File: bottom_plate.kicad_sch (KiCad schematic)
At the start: 27 parts, among them J42 Osc Out, J43 Conn_02x08_Odd_Even, J44 Conn_02x08_Odd_Even, J45 Conn_02x08_Odd_Even, J46 Conn_02x08_Odd_Even, J47 Conn_02x08_Odd_Even, J48 Select, J49 Select, J60 VCC, J61 VCC, J62 GND, J63 GND, J64 Conn_02x08_Odd_Even, J66 4017 Pins, J67 4017 Pins, J68 Conn_01x16, J73 Conn_02x20_Odd_Even, J74 Conn_02x20_Odd_Even, J75 Conn_02x20_Odd_Even, J76 Conn_02x20_Odd_Even, J77 Conn_02x20_Odd_Even, J78 Conn_02x20_Odd_Even, J79 Conn_02x20_Odd_Even, J80 Conn_02x20_Odd_Even, J81 Conn_02x20_Odd_Even, J85 Output, J86 Output

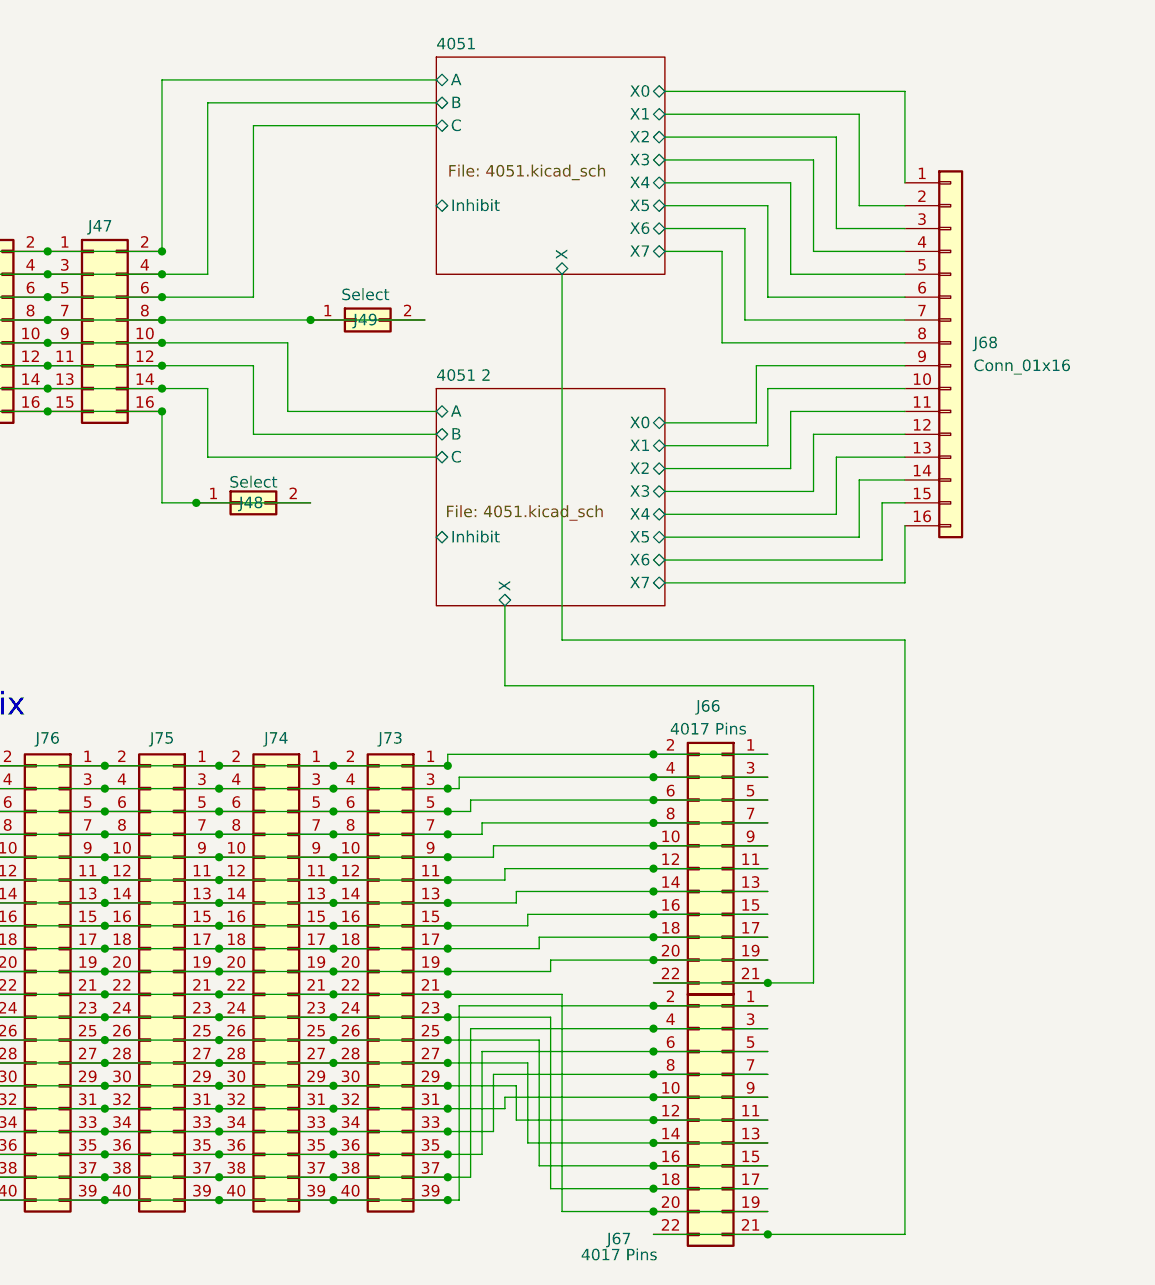
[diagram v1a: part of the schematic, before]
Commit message: 18x20 design
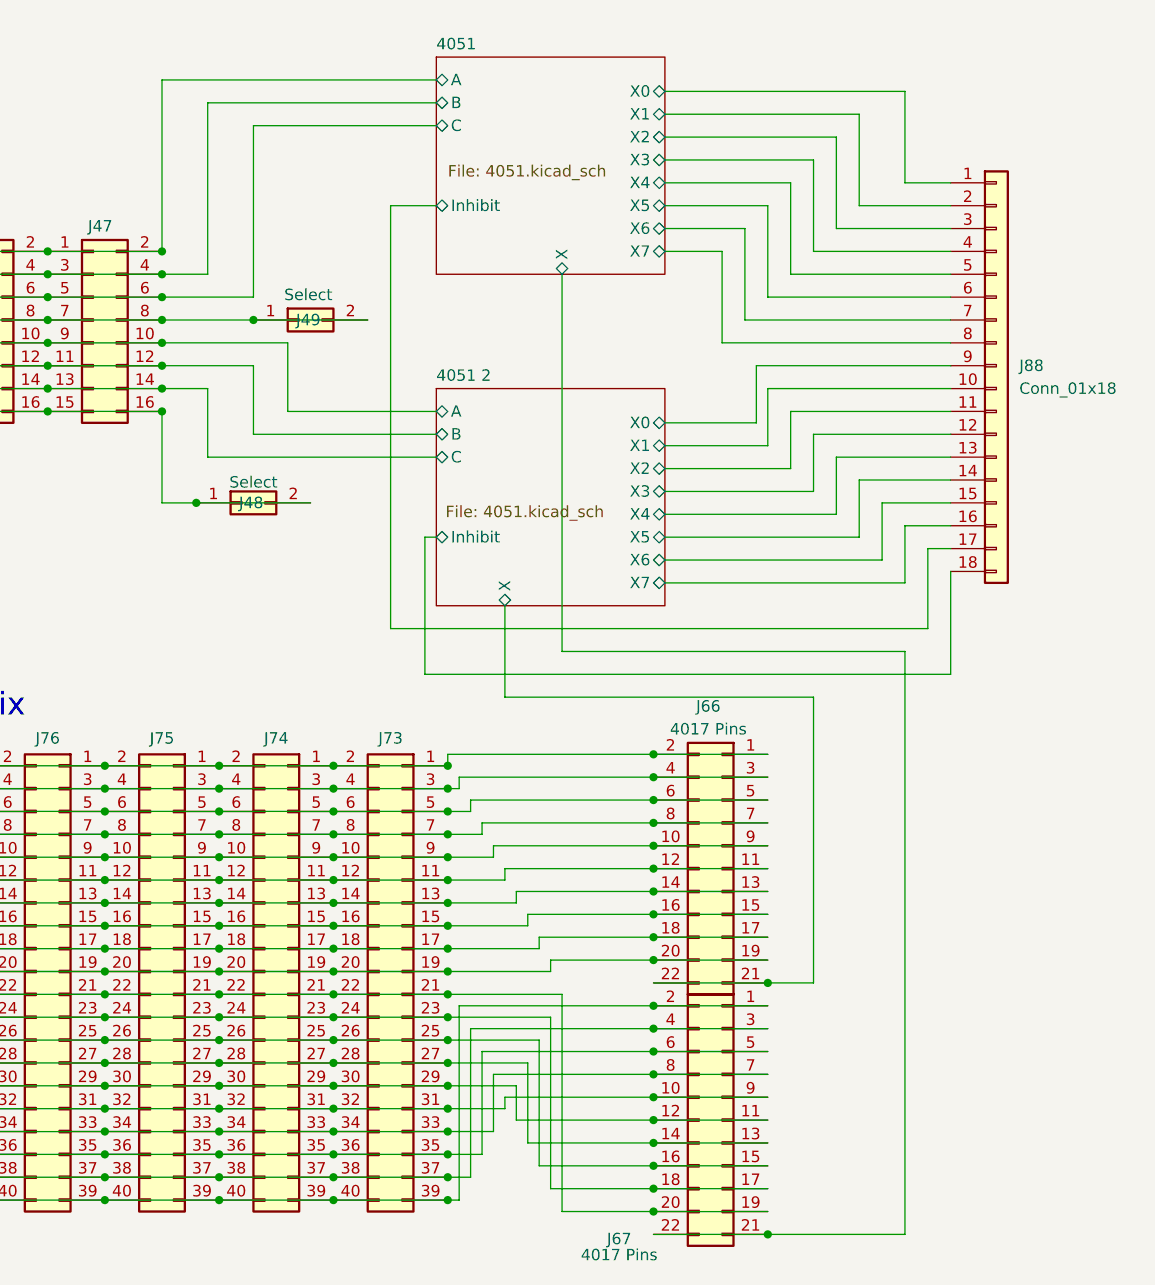
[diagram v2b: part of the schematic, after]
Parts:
- removed J68: Conn_01x16, Connector_PinSocket_2.54mm:PinSocket_1x16_P2.54mm_Vertical, symbol Connector_Generic:Conn_01x16
- added J88: Conn_01x18, Connector_PinHeader_2.54mm:PinHeader_1x18_P2.54mm_Vertical, symbol Connector_Generic:Conn_01x18
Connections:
- net 4051 2/Inhibit: now also J88.18 (Pin_18)
- net 4051 2/X0: now also J88.9 (Pin_9)
- net 4051 2/X1: now also J88.10 (Pin_10)
- net 4051 2/X2: now also J88.11 (Pin_11)
- net 4051 2/X3: now also J88.12 (Pin_12)
- net 4051 2/X4: now also J88.13 (Pin_13)
- net 4051 2/X5: now also J88.14 (Pin_14)
- net 4051 2/X6: now also J88.15 (Pin_15)
- net 4051 2/X7: now also J88.16 (Pin_16)
- net 4051/Inhibit: now also J88.17 (Pin_17)
- net 4051/X0: now also J88.1 (Pin_1)
- net 4051/X1: now also J88.2 (Pin_2)
- net 4051/X2: now also J88.3 (Pin_3)
- net 4051/X3: now also J88.4 (Pin_4)
- net 4051/X4: now also J88.5 (Pin_5)
- net 4051/X5: now also J88.6 (Pin_6)
- net 4051/X6: now also J88.7 (Pin_7)
- net 4051/X7: now also J88.8 (Pin_8)
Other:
- moved on the sheet: J49
